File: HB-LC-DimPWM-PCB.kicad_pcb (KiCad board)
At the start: 2 copper layers, 184 parts, among them J1 SWD, J3 Conn_01x04_Male, J4 Conn_01x04_Male, J5 Conn_01x04_Male, J6 Conn_01x04_Male, Q1 S9013, Q10 BSS84, Q11 2N7002, Q12 BSS84, Q13 2N7002, Q14 VS5810AS, Q15 VS5810AS, Q16 VS5810AS, Q17 VS5810AS, Q18 VS5810AS, Q19 VS5810AS, Q2 BSS84, Q20 VS5810AS, Q21 VS5810AS, Q22 VS5810AS, Q23 VS5810AS, Q24 VS5810AS, Q25 VS5810AS, Q26 VS5810AS, Q27 VS5810AS, Q28 VS5810AS, Q3 2N7002, Q4 VS5810AS, Q5 S9013, Q6 S9013, Q7 S9013, Q8 BSS84, Q9 2N7002, U1 STM32F103C8Tx, U10 MCP1416, U11 MCP1416, U12 MCP1416, U13 MCP1416, U14 MCP1416, U2 AMS1117-3.3, U3 MCP1416, U4 MCP1416, U5 MCP1416, U6 MCP1416, U7 MCP1416, U8 MCP1416, U9 MCP1416, Y1 8MHz

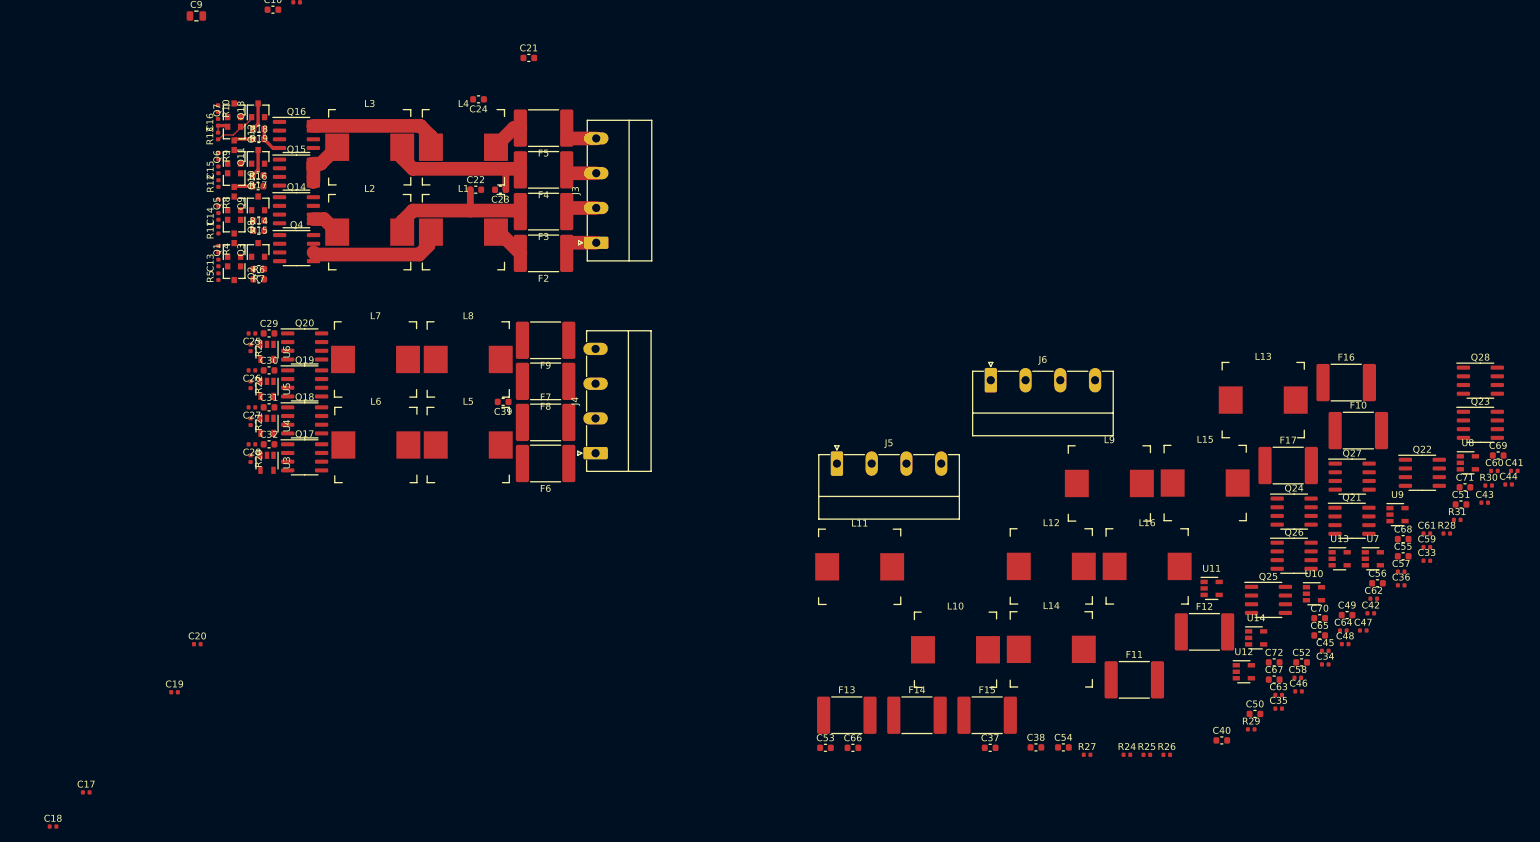
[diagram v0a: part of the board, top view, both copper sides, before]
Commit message: Layout one dimmer channel
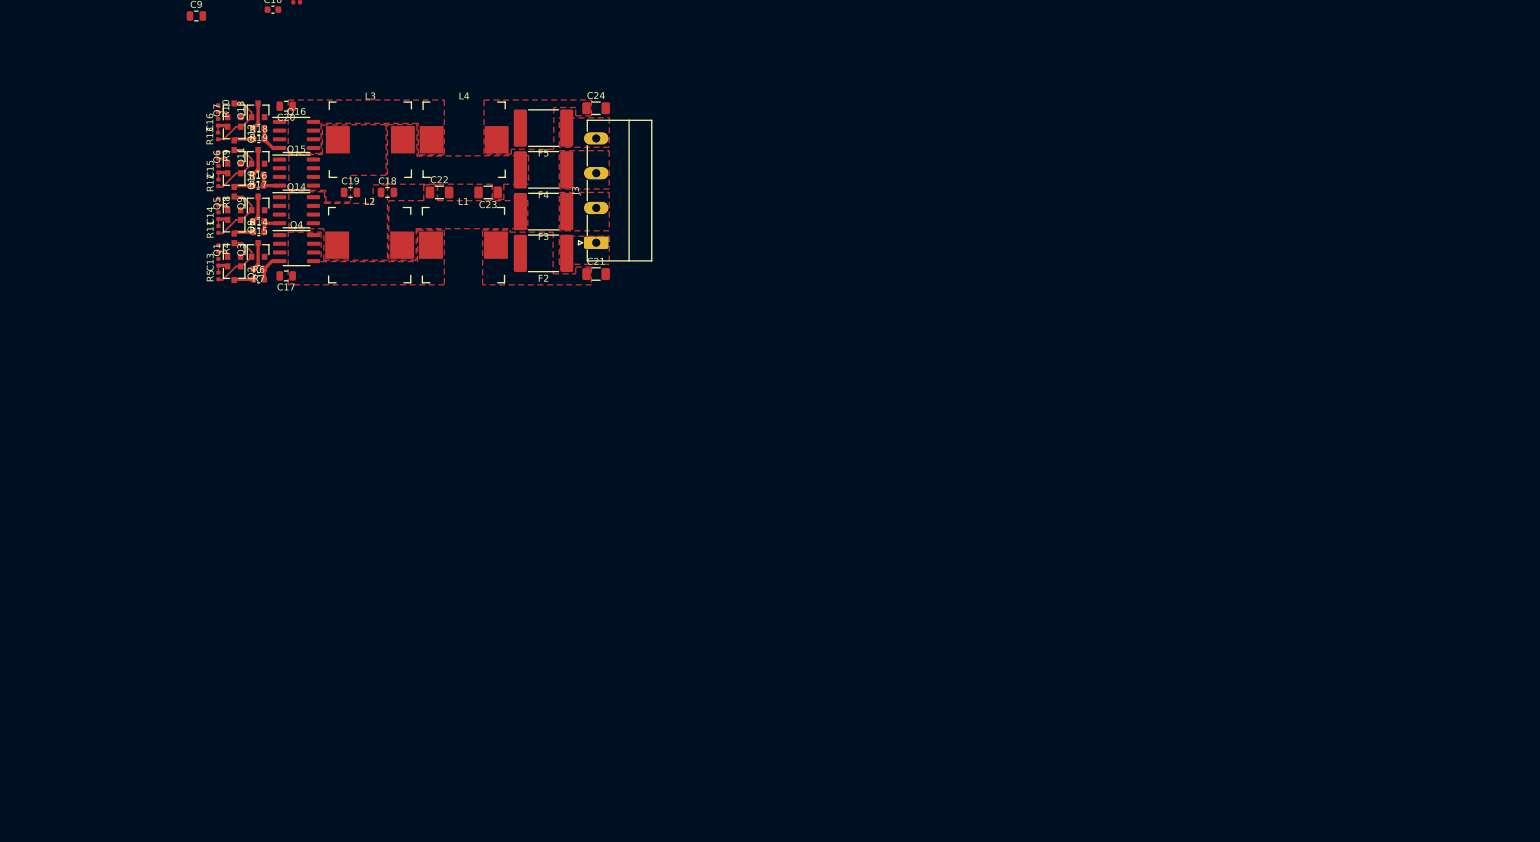
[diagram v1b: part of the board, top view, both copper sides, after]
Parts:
- removed C25, C26, C27, C28, C41, C42, C43, C44, C45, C46, C47, C48: 1uF, Capacitor_SMD:C_0402_1005Metric
- removed C29, C30, C31, C32, C49, C50, C51, C52, C53, C54, C55, C56: 100n, Capacitor_SMD:C_0603_1608Metric
- removed C33, C34, C35, C36, C57, C58, C59, C60, C61, C62, C63, C64: 100p, Capacitor_SMD:C_0402_1005Metric
- removed C37, C38, C39, C40, C65, C66, C67, C68, C69, C70, C71, C72: 1uF, Capacitor_SMD:C_0603_1608Metric
- removed F10, F11, F12, F13, F14, F15, F16, F17, F6, F7, F8, F9: 15V 5A, Fuse:Fuse_2920_7451Metric
- removed J4, J5, J6: Conn_01x04_Male, Connector_Phoenix_MC_HighVoltage:PhoenixContact_MC_1,5_4-G-5.08_1x04_P5.08mm_Horizontal
- removed L10, L11, L12, L13, L14, L15, L16, L5, L6, L7, L8, L9: 3.3uH, Inductor_Sunlord:SMD-PIND-10.5x11.5x4_2.5x3.0
- removed Q17, Q18, Q19, Q20, Q21, Q22, Q23, Q24, Q25, Q26, Q27, Q28: VS5810AS, Package_SO:SOIC-8_3.9x4.9mm_P1.27mm
- removed R20, R21, R22, R23, R24, R25, R26, R27, R28, R29, R30, R31: 10k, Resistor_SMD:R_0402_1005Metric
- removed U10, U11, U12, U13, U14, U3, U4, U5, U6, U7, U8, U9: MCP1416, Package_TO_SOT_SMD:SOT-23-5
- C17, C18, C19, C20: footprint Capacitor_SMD:C_0402_1005Metric -> Capacitor_SMD:C_0805_2012Metric
- C21, C22, C23, C24: footprint Capacitor_SMD:C_0603_1608Metric -> Capacitor_SMD:C_1206_3216Metric
- moved C18 104.7 mm to (134.7, 80.4)
- moved C17 80.9 mm to (119.9, 92.6), turned to 180 degrees
- moved C20 79.7 mm to (119.9, 67.8), turned to 180 degrees
- moved C19 77.4 mm to (129.3, 80.4)
- moved C21 33.1 mm to (165.2, 92.3)
- moved C24 17.2 mm to (165.2, 68.1), turned to 0 degrees
- moved C22 5.32 mm to (142.3, 80.4)
- moved L1 1.90 mm to (145.8, 88.1)
- moved L2 1.90 mm to (132.1, 88.1)
- moved C23 1.84 mm to (149.4, 80.4)
- moved L3 1.10 mm to (132.2, 72.7)
- moved L4 1.10 mm to (145.9, 72.7)
- moved R14 0.20 mm to (115.9, 86.2)
- moved C13 0.10 mm to (110.0, 90.6)
- moved C14 0.10 mm to (110.0, 83.8)
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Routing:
- net Net-(C22-Pad1): track 22.5 -> 0.00 mm
- net Net-(C23-Pad1): track 23.6 -> 1.12 mm
- net Net-(C17-Pad1): track 19.5 -> 0.00 mm
- net Net-(C20-Pad1): track 19.4 -> 0.00 mm
- net Net-(Q5-Pad3): track 0.00 -> 10.0 mm
- net Net-(Q1-Pad3): track 0.00 -> 10.0 mm
- net Net-(Q10-Pad1): track 0.00 -> 10.0 mm
- net +12V: track 2.49 -> 9.78 mm
- net Net-(C19-Pad1): track 6.68 -> 0.00 mm
- net Net-(C24-Pad1): track 4.83 -> 0.00 mm
- net Net-(C21-Pad1): track 4.64 -> 0.00 mm
- net Net-(Q4-Pad4): track 0.00 -> 4.24 mm
- net Net-(C18-Pad1): track 4.24 -> 0.00 mm
- net Net-(F2-Pad1): track 4.22 -> 0.00 mm
- net Net-(F5-Pad1): track 4.20 -> 0.00 mm
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- added copper zone on F.Cu, net Net-(C17-Pad1)
- added copper zone on F.Cu, net Net-(C18-Pad1)
- added copper zone on F.Cu, net Net-(C19-Pad1)
- added copper zone on F.Cu, net Net-(C20-Pad1)
- added copper zone on F.Cu, net Net-(C21-Pad1)
- added copper zone on F.Cu, net Net-(C22-Pad1)
- added copper zone on F.Cu, net Net-(C23-Pad1)
- added copper zone on F.Cu, net Net-(C24-Pad1)
- added copper zone on F.Cu, net Net-(F2-Pad1)
- added copper zone on F.Cu, net Net-(F3-Pad1)
- added copper zone on F.Cu, net Net-(F4-Pad1)
- added copper zone on F.Cu, net Net-(F5-Pad1)
